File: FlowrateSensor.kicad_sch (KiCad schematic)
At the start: 5 parts, among them Q3 BUK7M27-80EX

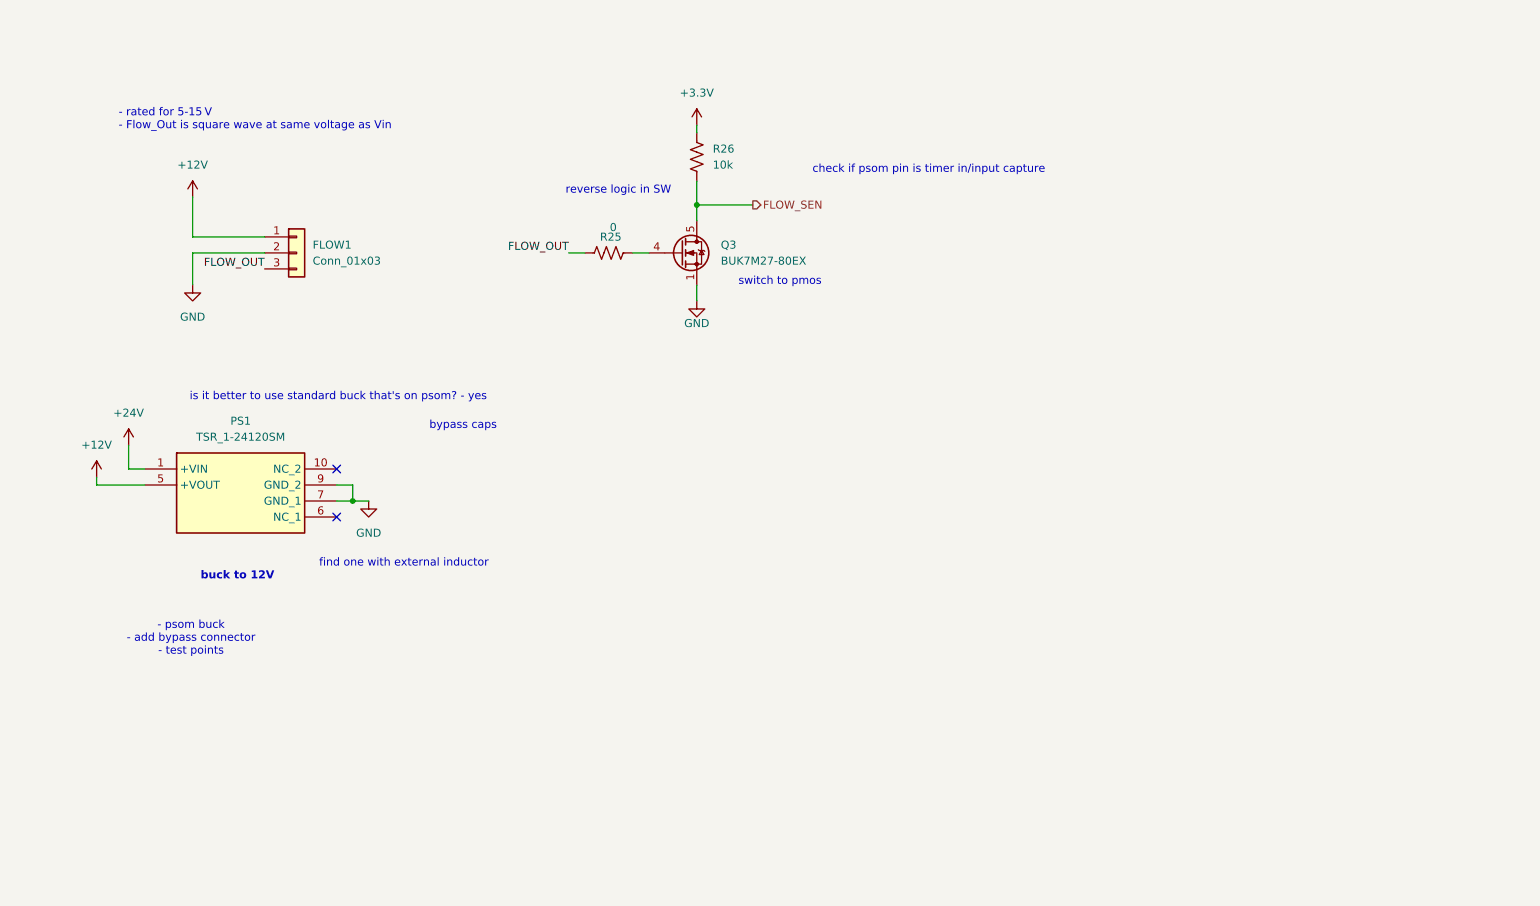
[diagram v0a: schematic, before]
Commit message: schematic changes before switching submodules
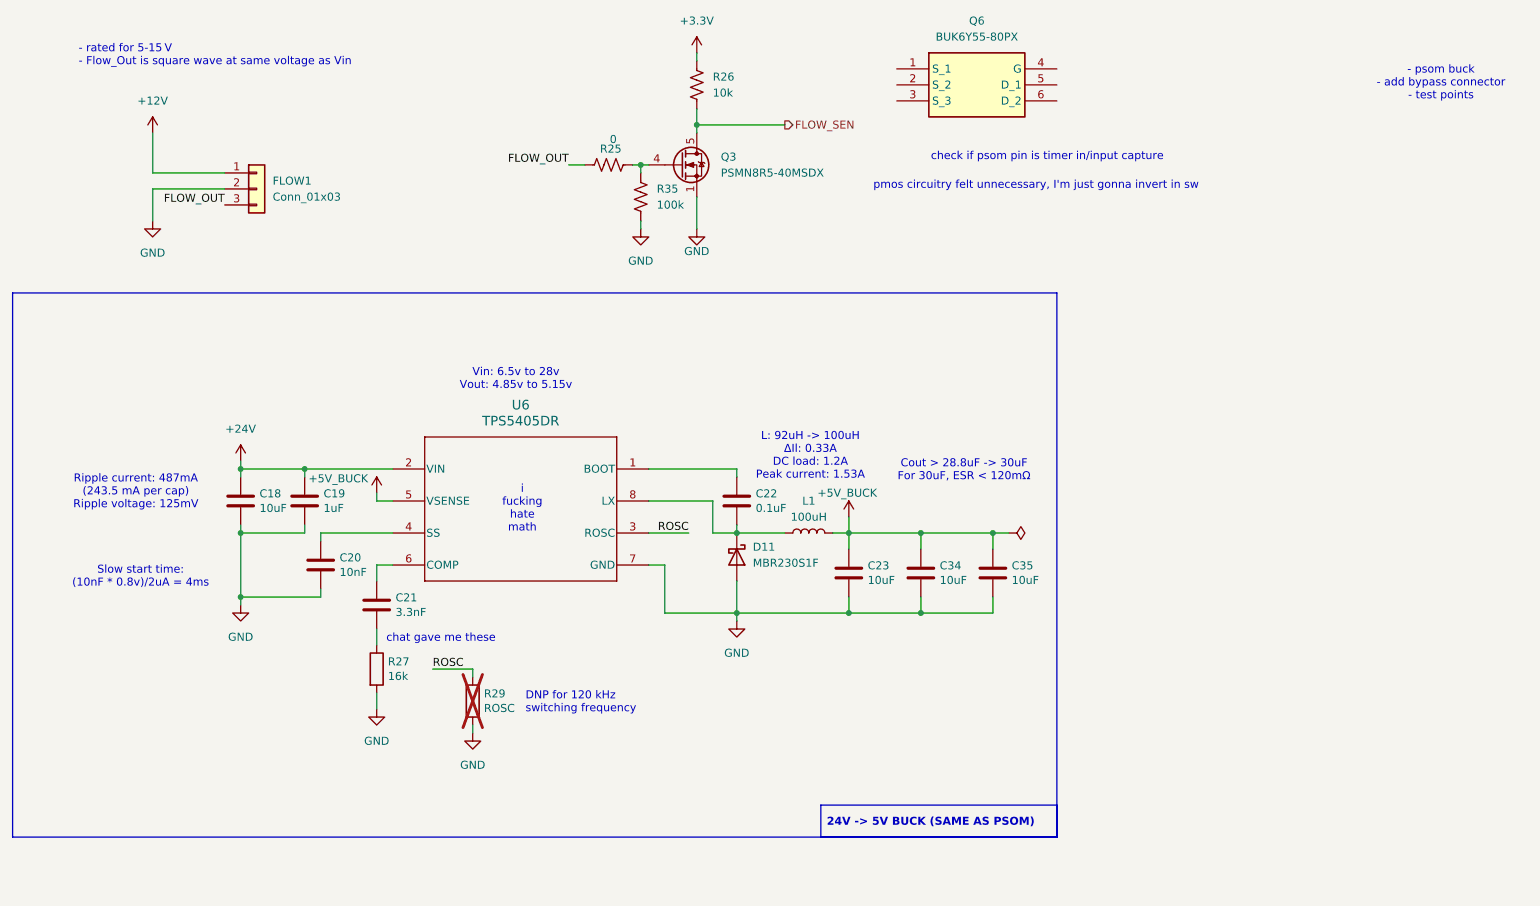
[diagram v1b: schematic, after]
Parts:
- removed PS1: TSR_1-24120SM, TSR_1-24120SM:TSR124120SM, symbol TSR_1-24120SM:TSR_1-24120SM
- added C18, C23, C34, C35: 10uF, Capacitor_SMD:C_0805_2012Metric_Pad1.18x1.45mm_HandSolder, symbol Device:C
- added C19: 1uF, Capacitor_SMD:C_0603_1608Metric_Pad1.08x0.95mm_HandSolder, symbol Device:C
- added C20: 10nF, Capacitor_SMD:C_0603_1608Metric_Pad1.08x0.95mm_HandSolder, symbol Device:C
- added C21: 3.3nF, Capacitor_SMD:C_0603_1608Metric_Pad1.08x0.95mm_HandSolder, symbol Device:C
- added C22: 0.1uF, Capacitor_SMD:C_0603_1608Metric_Pad1.08x0.95mm_HandSolder, symbol Device:C
- added D11: MBR230S1F, Diode_SMD:D_SOD-123F, symbol Device:D_Schottky
- added L1: 100uH, Inductor_SMD:L_Coilcraft_MSS1246-XXX, symbol Device:L
- added Q6: BUK6Y55-80PX, BUK6Y55-80PX:PHPT61002NYCLHX, symbol BUK6Y55-80PX:BUK6Y55-80PX
- added R27: 16k, Resistor_SMD:R_0603_1608Metric_Pad0.98x0.95mm_HandSolder, symbol Device:R
- added R29: ROSC, Resistor_SMD:R_0603_1608Metric_Pad0.98x0.95mm_HandSolder, symbol Device:R
- added R35: 100k, Resistor_SMD:R_0603_1608Metric, symbol Device:R_US
- added U6: TPS5405DR, UTSVT_Power:TPS5405DR, symbol utsvt_power:TPS5405DR
- Q3: value BUK7M27-80EX -> PSMN8R5-40MSDX
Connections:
- net +24V: now also C18.1, C19.1, U6.2 (VIN)
- net GND: now also C18.2, C19.2, C20.2, C23.2, C34.2, C35.2, D11.2 (A), R27.2, R29.2, R35.2, U6.7 (GND)
- net at Q3.4 (G), R25.2: now also R35.1
- new net: C22.1, U6.1 (BOOT)
- new net: C22.2, D11.1 (K), L1.1, U6.8 (LX)
- new net: C20.1, U6.4 (SS)
- new net: C21.1, U6.6 (COMP)
- new net: C21.2, R27.1
- new net +5V_BUCK: C23.1, C34.1, C35.1, L1.2, U6.5 (VSENSE)
- new net ROSC: R29.1, U6.3 (ROSC)
- no-connect marks 2 -> 0
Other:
- note added: "Cout > 28.8uF -> 30uF For 30uF, ESR < 120mΩ"
- note added: "DNP for 120 kHz switching frequency"
- note added: "L: 92uH -> 100uH ΔIl: 0.33A DC load: 1.2A Peak current: 1.53A"
- note added: "Ripple current: 487mA (243.5 mA per cap) Ripple voltage: 125mV"
- note added: "Slow start time: (10nF * 0.8v)/2uA = 4ms"
- note added: "Vin: 6.5v to 28v Vout: 4.85v to 5.15v"
- note added: "chat gave me these"
- note added: "i fucking hate math"
- note added: "pmos circuitry felt unnecessary, I'm just gonna invert in sw"
- note removed: "buck to 12V"
- note removed: "bypass caps"
- note removed: "find one with external inductor"
- note removed: "is it better to use standard buck that's on psom? - yes"
- note removed: "reverse logic in SW"
- note removed: "switch to pmos"
- moved on the sheet: FLOW1, R25, R26

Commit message: fixed submodule, schematic basically done
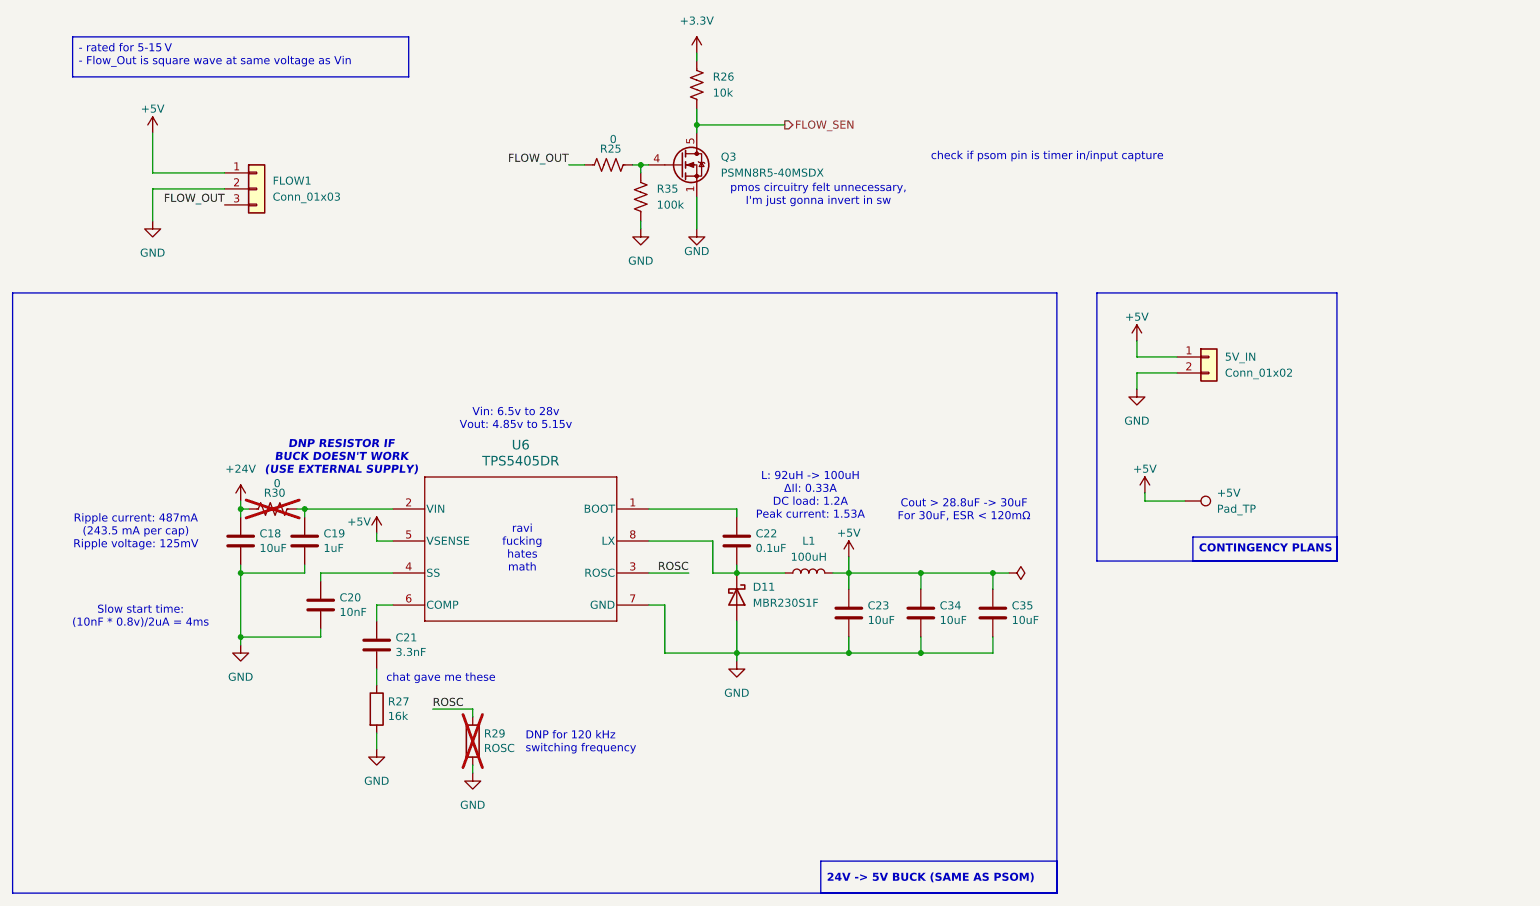
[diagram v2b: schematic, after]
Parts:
- removed Q6: BUK6Y55-80PX, BUK6Y55-80PX:PHPT61002NYCLHX, symbol BUK6Y55-80PX:BUK6Y55-80PX
- added +5V: Pad_TP, UTSVT_Special:TestPoint_HEX_3mmID, symbol Connector:TestPoint
- added 5V_IN: Conn_01x02, UTSVT_Connectors:Molex_Nano-Fit_105309-xx02_1x02_P2.50mm_Vertical, symbol Connector_Generic:Conn_01x02
- added R30: 0, Resistor_SMD:R_0603_1608Metric, symbol Device:R_US
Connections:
- net +5V_BUCK is gone; now on net +5V: C23.1, C34.1, C35.1, L1.2, U6.5 (VSENSE)
- net +24V: now also R30.1; no longer C19.1, U6.2 (VIN)
- net GND: now also 5V_IN.2 (Pin_2)
- net +12V renamed +5V
- net +5V: now also +5V.1, 5V_IN.1 (Pin_1)
- new net: C19.1, R30.2, U6.2 (VIN)
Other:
- note added: "DNP RESISTOR IF BUCK DOESN'T WORK (USE EXTERNAL SUPPLY)"
- note added: "ravi fucking hates math"
- note removed: "- psom buck - add bypass connector - test points"
- note removed: "i fucking hate math"
- moved on the sheet: C18, C19, C20, C21, C22, C23, C34, C35, D11, L1, R27, R29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
